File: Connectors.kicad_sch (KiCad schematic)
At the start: 6 parts, among them J1 MAIN, J2 PRG CONN

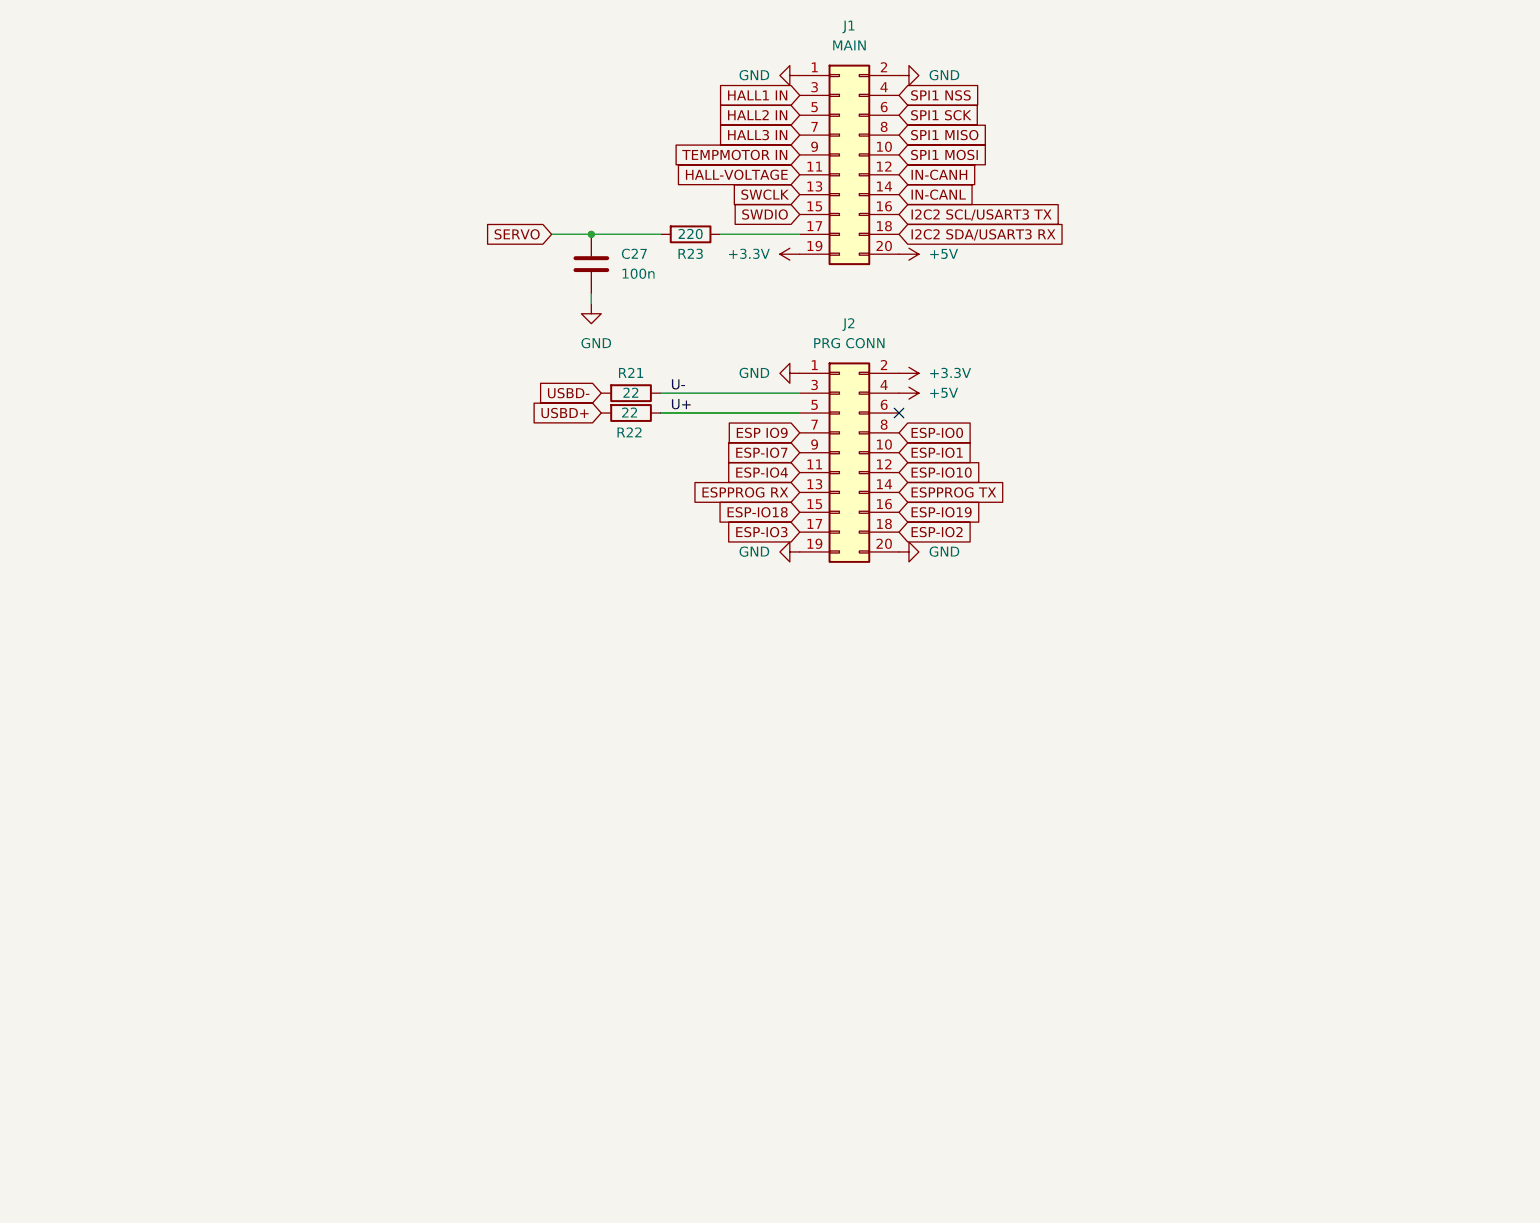
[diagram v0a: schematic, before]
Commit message: initial
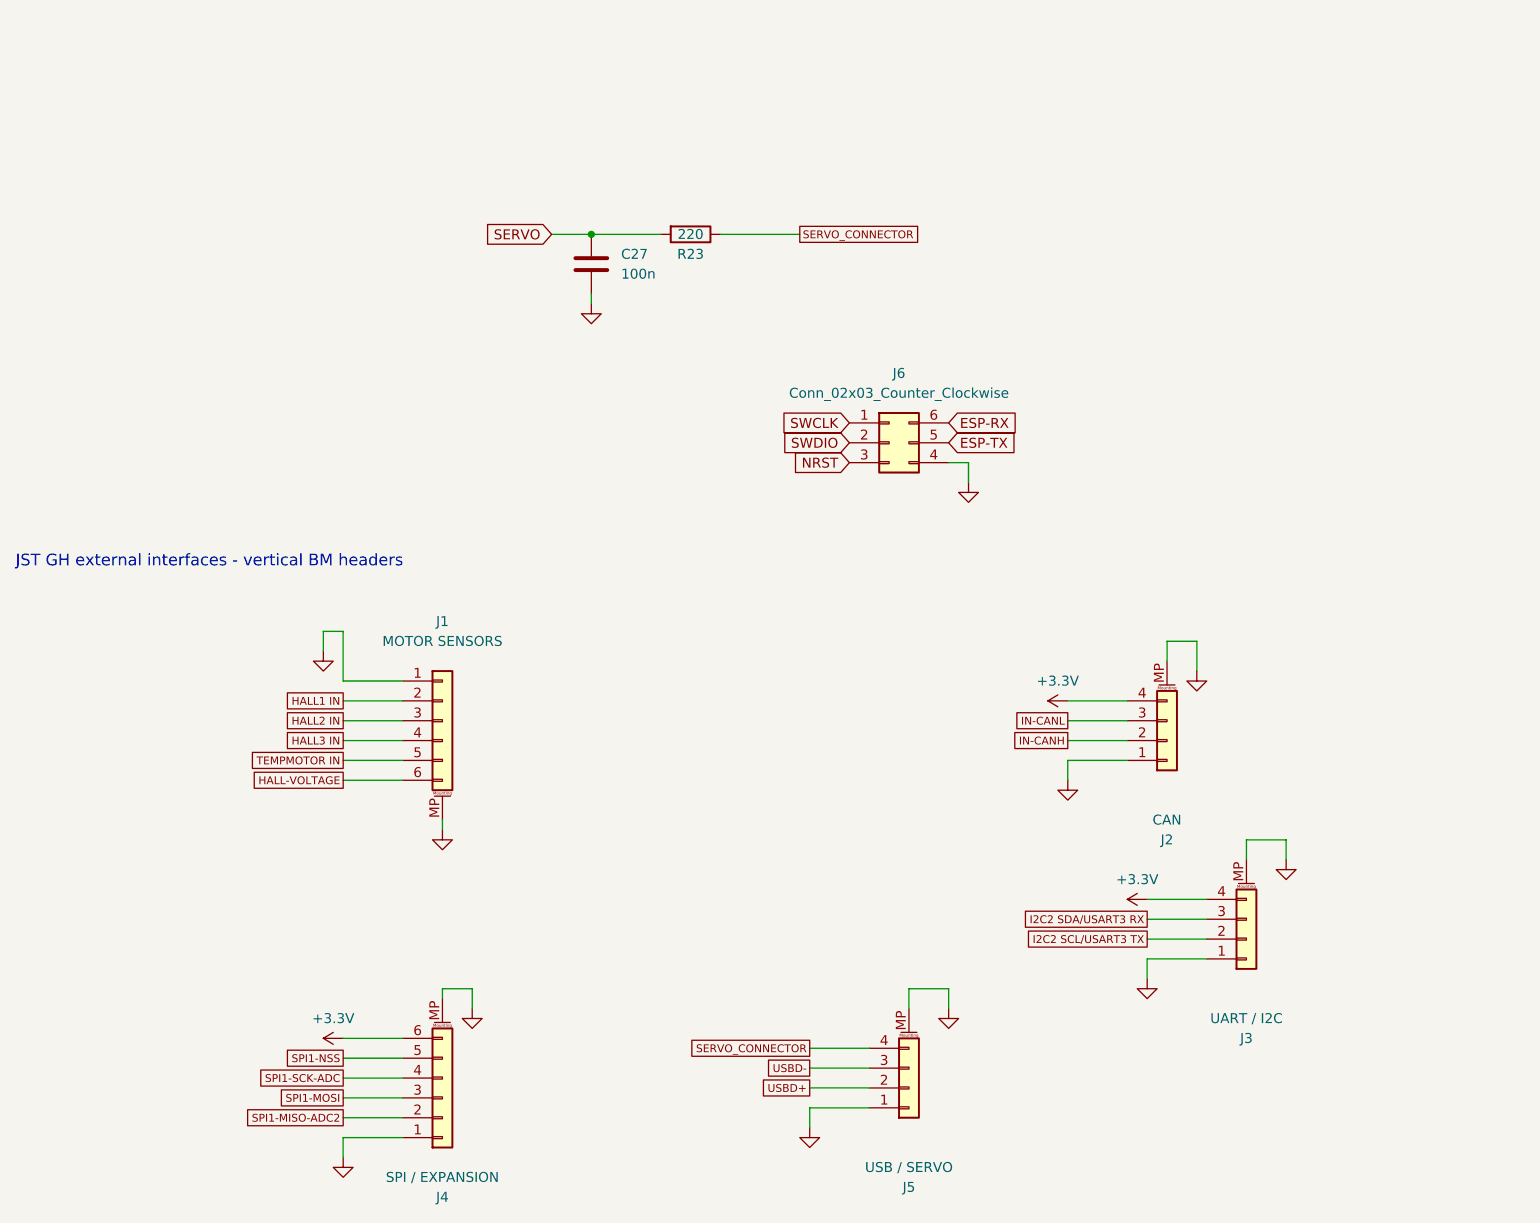
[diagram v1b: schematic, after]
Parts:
- removed J1: MAIN, Connector_JST:JST_PHD_B20B-PHDSS_2x10_P2.00mm_Vertical, symbol Connector_Generic:Conn_02x10_Odd_Even
- removed J2: PRG CONN, Connector_JST:JST_PHD_B20B-PHDSS_2x10_P2.00mm_Vertical, symbol Connector_Generic:Conn_02x10_Odd_Even
- removed R21, R22: 22, Resistor_SMD:R_0603_1608Metric, symbol Device:R
- added J1: MOTOR SENSORS, Connector_JST:JST_GH_BM06B-GHS-TBT_1x06-1MP_P1.25mm_Vertical, symbol Connector_Generic_MountingPin:Conn_01x06_MountingPin
- added J2: CAN, Connector_JST:JST_GH_BM04B-GHS-TBT_1x04-1MP_P1.25mm_Vertical, symbol Connector_Generic_MountingPin:Conn_01x04_MountingPin
- added J3: UART / I2C, Connector_JST:JST_GH_BM04B-GHS-TBT_1x04-1MP_P1.25mm_Vertical, symbol Connector_Generic_MountingPin:Conn_01x04_MountingPin
- added J4: SPI / EXPANSION, Connector_JST:JST_GH_BM06B-GHS-TBT_1x06-1MP_P1.25mm_Vertical, symbol Connector_Generic_MountingPin:Conn_01x06_MountingPin
- added J5: USB / SERVO, Connector_JST:JST_GH_BM04B-GHS-TBT_1x04-1MP_P1.25mm_Vertical, symbol Connector_Generic_MountingPin:Conn_01x04_MountingPin
- added J6: Conn_02x03_Counter_Clockwise, Connector_PinHeader_1.00mm:PinHeader_2x03_P1.00mm_Vertical, symbol Connector_Generic:Conn_02x03_Counter_Clockwise
- C27: footprint Capacitor_SMD:C_0603_1608Metric -> Capacitor_SMD:C_0402_1005Metric; MPN C14663 -> C1525
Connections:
- net +3.3V: now also J2.4 (Pin_4), J3.4 (Pin_4), J4.6 (Pin_6)
- net GND: now also J1.1 (Pin_1), J1.MP (MountPin), J2.1 (Pin_1), J2.MP (MountPin), J3.1 (Pin_1), J3.MP (MountPin), J4.1 (Pin_1), J4.MP (MountPin), J5.1 (Pin_1), J5.MP (MountPin), J6.4 (Pin_4)
- net HALL-VOLTAGE: now also J1.6 (Pin_6)
- net HALL1 IN: now also J1.2 (Pin_2)
- net HALL2 IN: now also J1.3 (Pin_3)
- net HALL3 IN: now also J1.4 (Pin_4)
- net I2C2 SCL/USART3 TX: now also J3.2 (Pin_2)
- net I2C2 SDA/USART3 RX: now also J3.3 (Pin_3)
- net IN-CANH: now also J2.2 (Pin_2)
- net IN-CANL: now also J2.3 (Pin_3)
- net SWCLK: now also J6.1 (Pin_1)
- net SWDIO: now also J6.2 (Pin_2)
- net TEMPMOTOR IN: now also J1.5 (Pin_5)
- net USBD+: now also J5.2 (Pin_2)
- net USBD-: now also J5.3 (Pin_3)
- net SERVO_CONNECTOR: now reaches R23.1
- net SERVO_CONNECTOR: now also J5.4 (Pin_4)
- new net ESP-RX: J6.6 (Pin_6)
- new net ESP-TX: J6.5 (Pin_5)
- new net NRST: J6.3 (Pin_3)
- new net SPI1-MISO-ADC2: J4.2 (Pin_2)
- new net SPI1-MOSI: J4.3 (Pin_3)
- new net SPI1-NSS: J4.5 (Pin_5)
- new net SPI1-SCK-ADC: J4.4 (Pin_4)
- no-connect marks 1 -> 0
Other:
- note added: "JST GH external interfaces - vertical BM headers"

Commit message: gate resistors
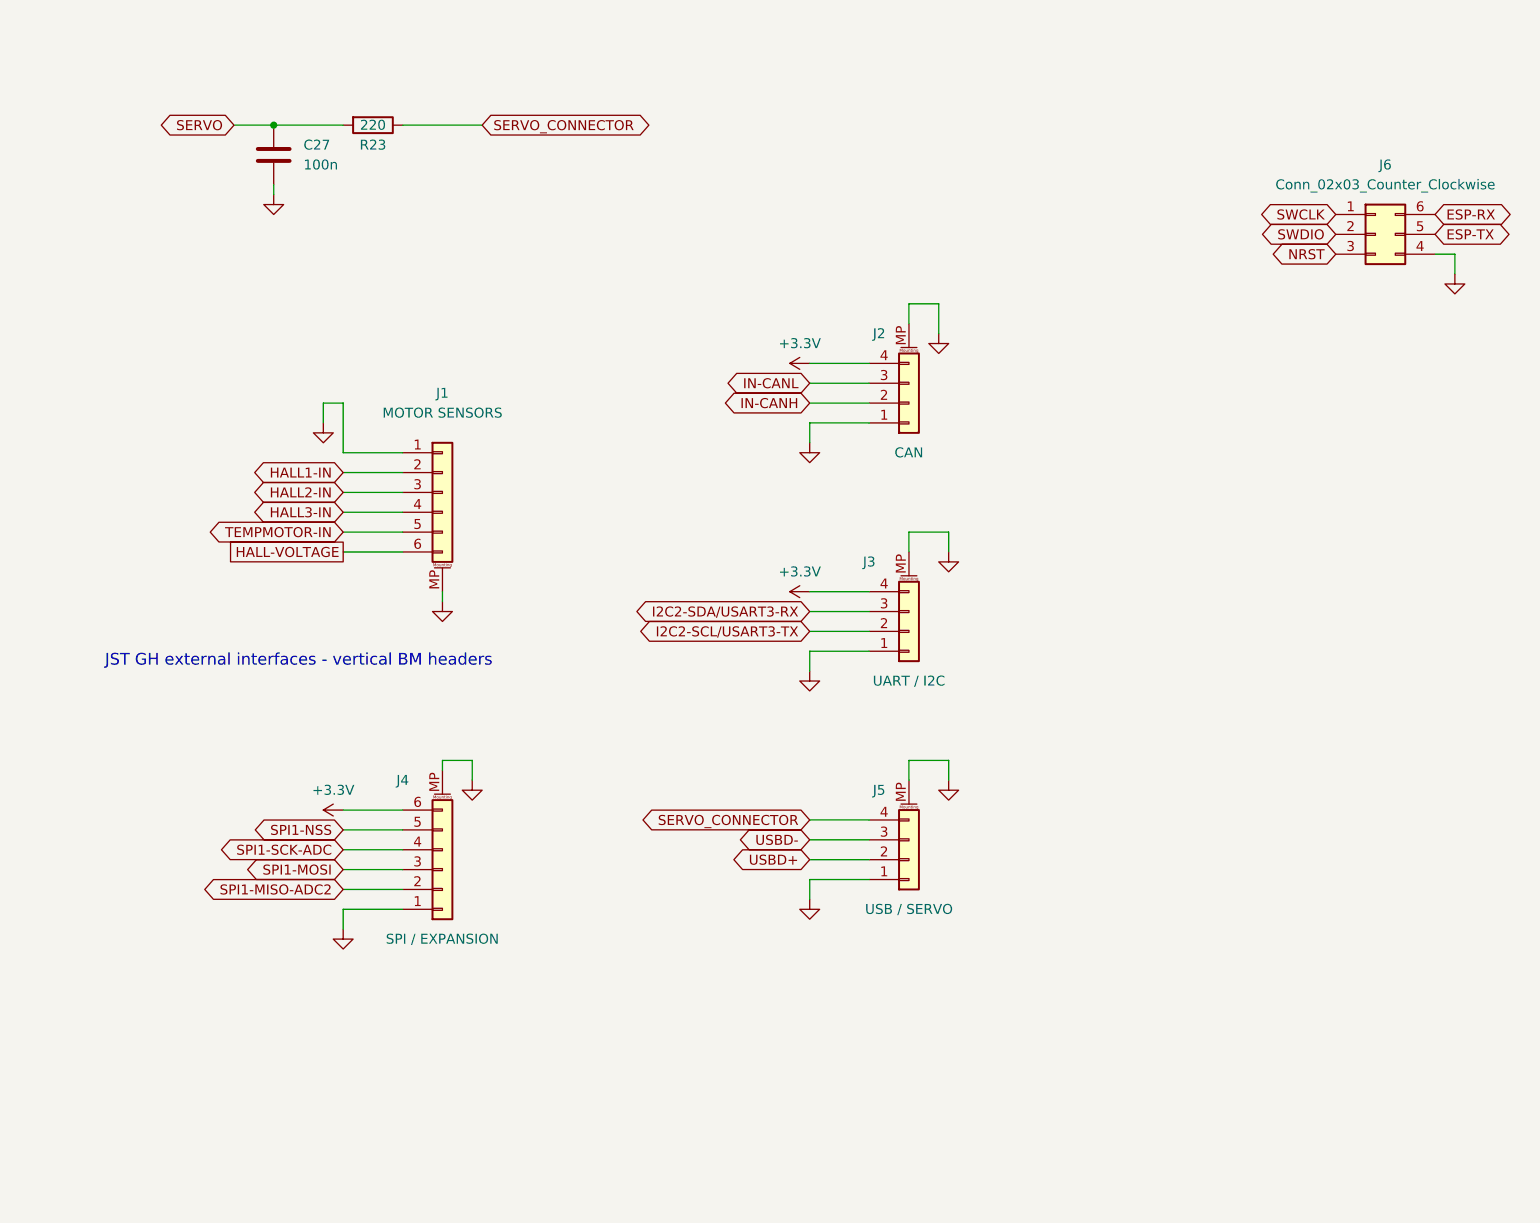
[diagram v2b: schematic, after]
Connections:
- net HALL1 IN renamed HALL1-IN
- net HALL2 IN renamed HALL2-IN
- net HALL3 IN renamed HALL3-IN
- net I2C2 SCL/USART3 TX renamed I2C2-SCL/USART3-TX
- net I2C2 SDA/USART3 RX renamed I2C2-SDA/USART3-RX
- net TEMPMOTOR IN renamed TEMPMOTOR-IN
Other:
- moved on the sheet: C27, J1, J2, J3, J4, J5, J6, R23
